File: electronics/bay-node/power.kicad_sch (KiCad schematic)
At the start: 26 parts, among them J1 24V IN, J2 24V OUT, Q1 SUD50P06-15, U1 TPS54360BDDAR, U2 AMS1117-3.3

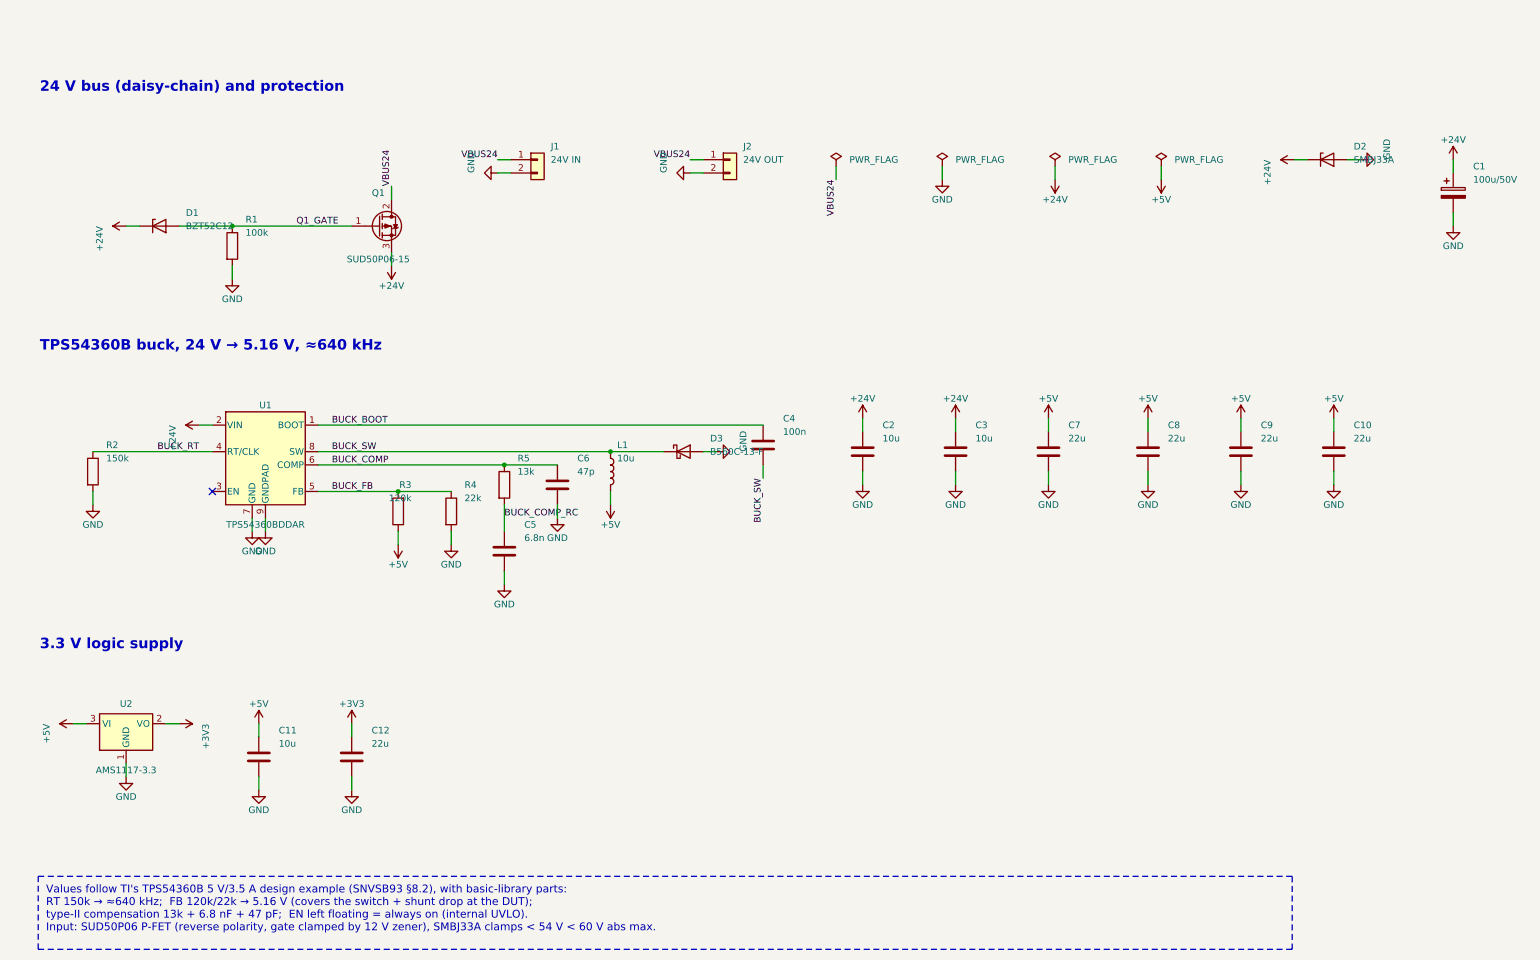
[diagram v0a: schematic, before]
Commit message: Boards v0.2: LMR51635 buck, JST PH, drawn schematics, thermal reliefs
Addresses Fabio's review of v0.1.

Bay node (rev 0.2):
- 5 V buck: LMR51635YDDCR (60 V, 3.5 A, synchronous, 1.1 MHz) with a
  3.3 uH FXL0630, 3 x 22 uF out, 2 x 10 uF + 100 nF in, FB 120k/22k
  (5.16 V), EN 1M/100k UVLO (13.5 V on, 10.8 V off). Replaces the
  TPS54360B, its Schottky and compensation network. CIN straddles the
  VIN/GND pins on solid top-side islands with vias to In1 (TI SLUSF64B).
- 24 V in/out on JST PH (carrier notches resized, rack.yaml pwr_y).
- Power nets named along the path: 24V_BUS -> +24V -> +5V -> DUT_5V_SW
  -> shunt -> DUT_5V; the INA226 visibly runs from +3V3.
- Stackup S+GND / GND / PWR / S+GND: In2 carries +5V, +3V3 under the
  ESP32 and a protected 24 V bus strip. Outer GND pours kept (without
  them Freerouting left ~25 connections unrouted).

Power hub (rev 0.2): JST VH input instead of the screw terminal, JST PH
row outputs, eFuse limit 1.6 A (RILIM 7.5k) to protect the 2 A contacts.

Generator:
- eda.py: drawn schematic mode (sch= placement, Sheet.wire/tag/frame,
  rotated/mirrored symbols, automatic junctions, per-island labels and
  checks that no wire touches another net); all seven sheets redrawn.
- pcbgen.py: thermal reliefs on every pour (+ <board>.kicad_dru for
  single spokes on fine pitch), configurable inner layers, per-zone
  deferral, fixed vias, DRC-driven fix-up for isolated GND pads.
- JLC CPL fix for the LMR51635 (270 deg); BOM, cables, viewer, docs.

ERC 0, DRC 0 copper errors, 0 unconnected, schematic parity 0 on both.

Co-Authored-By: Claude Opus 5.5 <noreply@anthropic.com>
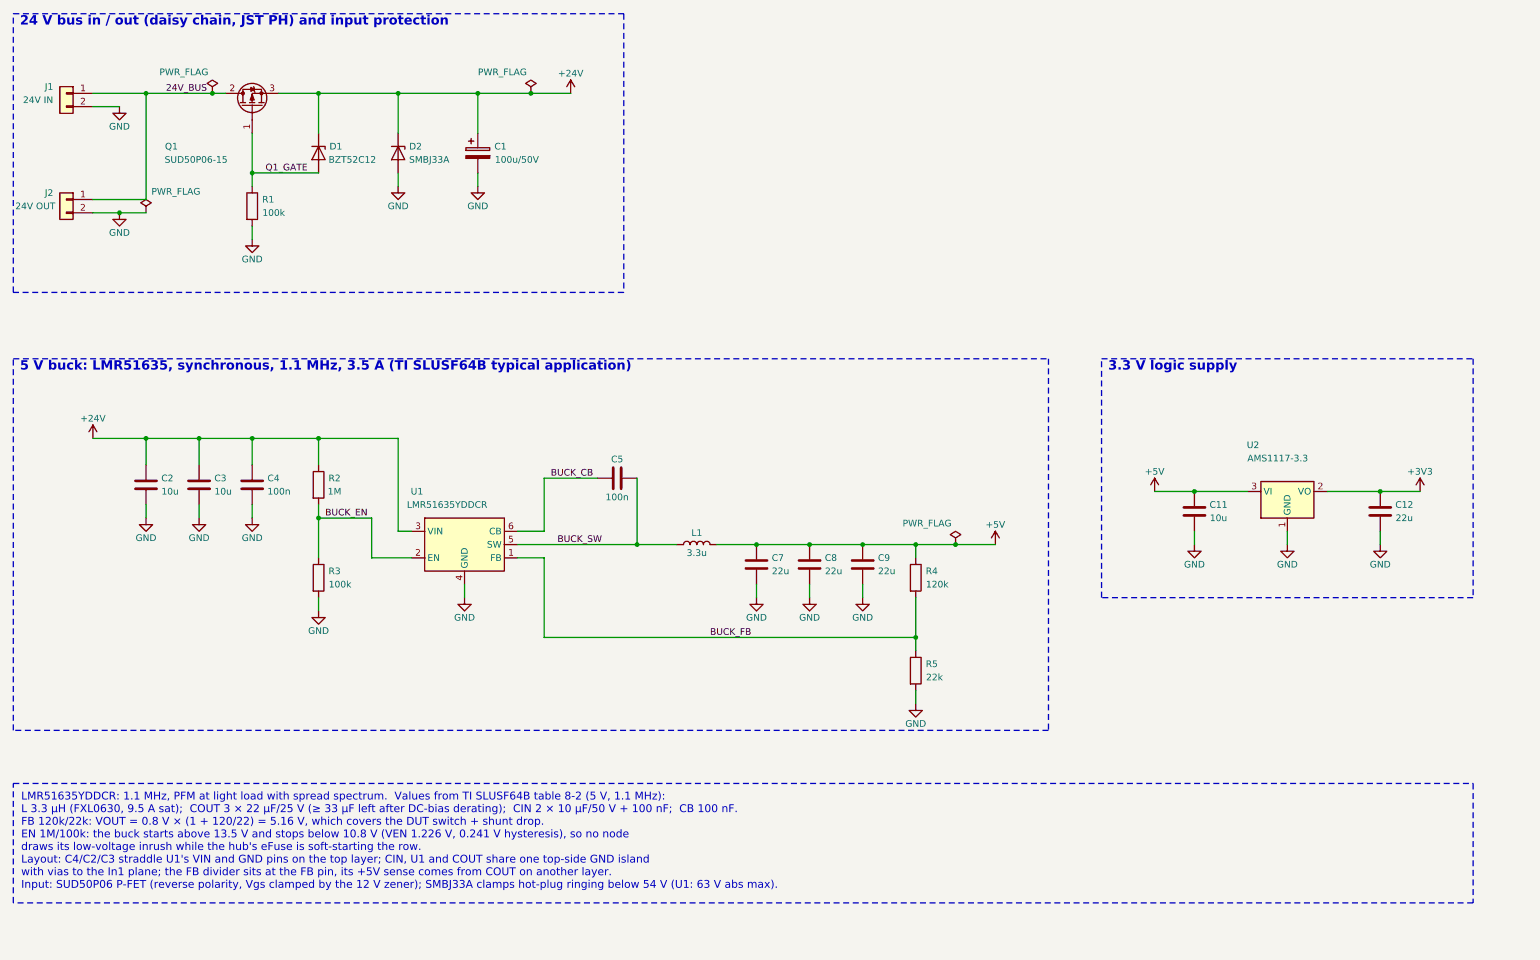
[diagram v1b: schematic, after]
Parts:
- removed C10: 22u, Capacitor_SMD:C_1206_3216Metric, symbol Device:C
- removed C6: 47p, Capacitor_SMD:C_0603_1608Metric, symbol Device:C
- removed D3: B560C-13-F, Diode_SMD:D_SMC, symbol Device:D_Schottky
- C5: value 6.8n -> 100n; LCSC C1631 -> C14663; MPN 0603B682K500NT -> CC0603KRX7R9BB104; Manufacturer FH (Guangdong Fenghua Advanced Tech) -> YAGEO
- J1, J2: footprint Connector_JST:JST_VH_S2P-VH_1x02_P3.96mm_Horizontal -> Connector_JST:JST_PH_S2B-PH-K_1x02_P2.00mm_Horizontal; LCSC C160355 -> C173752; MPN S2P-VH(LF)(SN) -> S2B-PH-K-S(LF)(SN)
- L1: value 10u -> 3.3u; footprint Inductor_SMD:L_Changjiang_FXL1040 -> Inductor_SMD:L_Changjiang_FXL0630; LCSC C475915 -> C167219; MPN FXL1040-100-M -> FXL0630-3R3-M
- R2: value 150k -> 1M; LCSC C22807 -> C22935; MPN 0603WAF1503T5E -> 0603WAF1004T5E
- R3: value 120k -> 100k; LCSC C25808 -> C25803; MPN 0603WAF1203T5E -> 0603WAF1003T5E
- R4: value 22k -> 120k; LCSC C31850 -> C25808; MPN 0603WAF2202T5E -> 0603WAF1203T5E
- R5: value 13k -> 22k; LCSC C22797 -> C31850; MPN 0603WAF1302T5E -> 0603WAF2202T5E
- U1: value TPS54360BDDAR -> LMR51635YDDCR; footprint Package_SO:TI_SO-PowerPAD-8_ThermalVias -> Package_TO_SOT_SMD:TSOT-23-6; symbol Regulator_Switching:TPS54360DDA -> bench:LMR51635; Alternative (none) -> LMR51635YFDDCR (C44750836): same, forced PWM, no spread spe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; LCSC C524806 -> C45262770; MPN TPS54360BDDAR -> LMR51635YDDCR
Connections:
- net +24V: now also C4.1, R2.1, U1.3 (VIN); no longer U1.2 (VIN)
- net +5V: now also R4.1; no longer R3.1
- net BUCK_FB: now also R4.2, R5.1, U1.1 (FB); no longer R3.2, R4.1, U1.5 (FB)
- net BUCK_SW: now also C5.2, U1.5 (SW); no longer C4.2, U1.8 (SW)
- net GND: now also C4.2, R3.2, R5.2, U1.4 (GND); no longer C5.2, R2.2, R4.2, U1.7 (GND), U1.9 (GNDPAD)
- removed net BUCK_BOOT: C4.1, U1.1 (BOOT)
- net BUCK_COMP renamed BUCK_CB
- net BUCK_CB: now also C5.1; no longer R5.1
- removed net BUCK_COMP_RC: C5.1, R5.2
- removed net BUCK_RT: R2.1, U1.4 (RT/CLK)
- net VBUS24 renamed 24V_BUS
- new net BUCK_EN: R2.2, R3.1, U1.2 (EN)
- no-connect marks 1 -> 0
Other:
- note added: "24 V bus in / out (daisy chain, JST PH) and input protection"
- note added: "5 V buck: LMR51635, synchronous, 1.1 MHz, 3.5 A (TI SLUSF64B typical application)"
- note removed: "24 V bus (daisy-chain) and protection"
- note removed: "TPS54360B buck, 24 V → 5.16 V, ≈640 kHz"
- moved on the sheet: C1, C11, C12, C2, C3, C4, C5, C7, C8, C9, D1, D2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
